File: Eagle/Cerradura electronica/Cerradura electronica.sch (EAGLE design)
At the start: 19 parts, among them K1 G5L, M1 ARDUINO-NANO-3.0#ISP

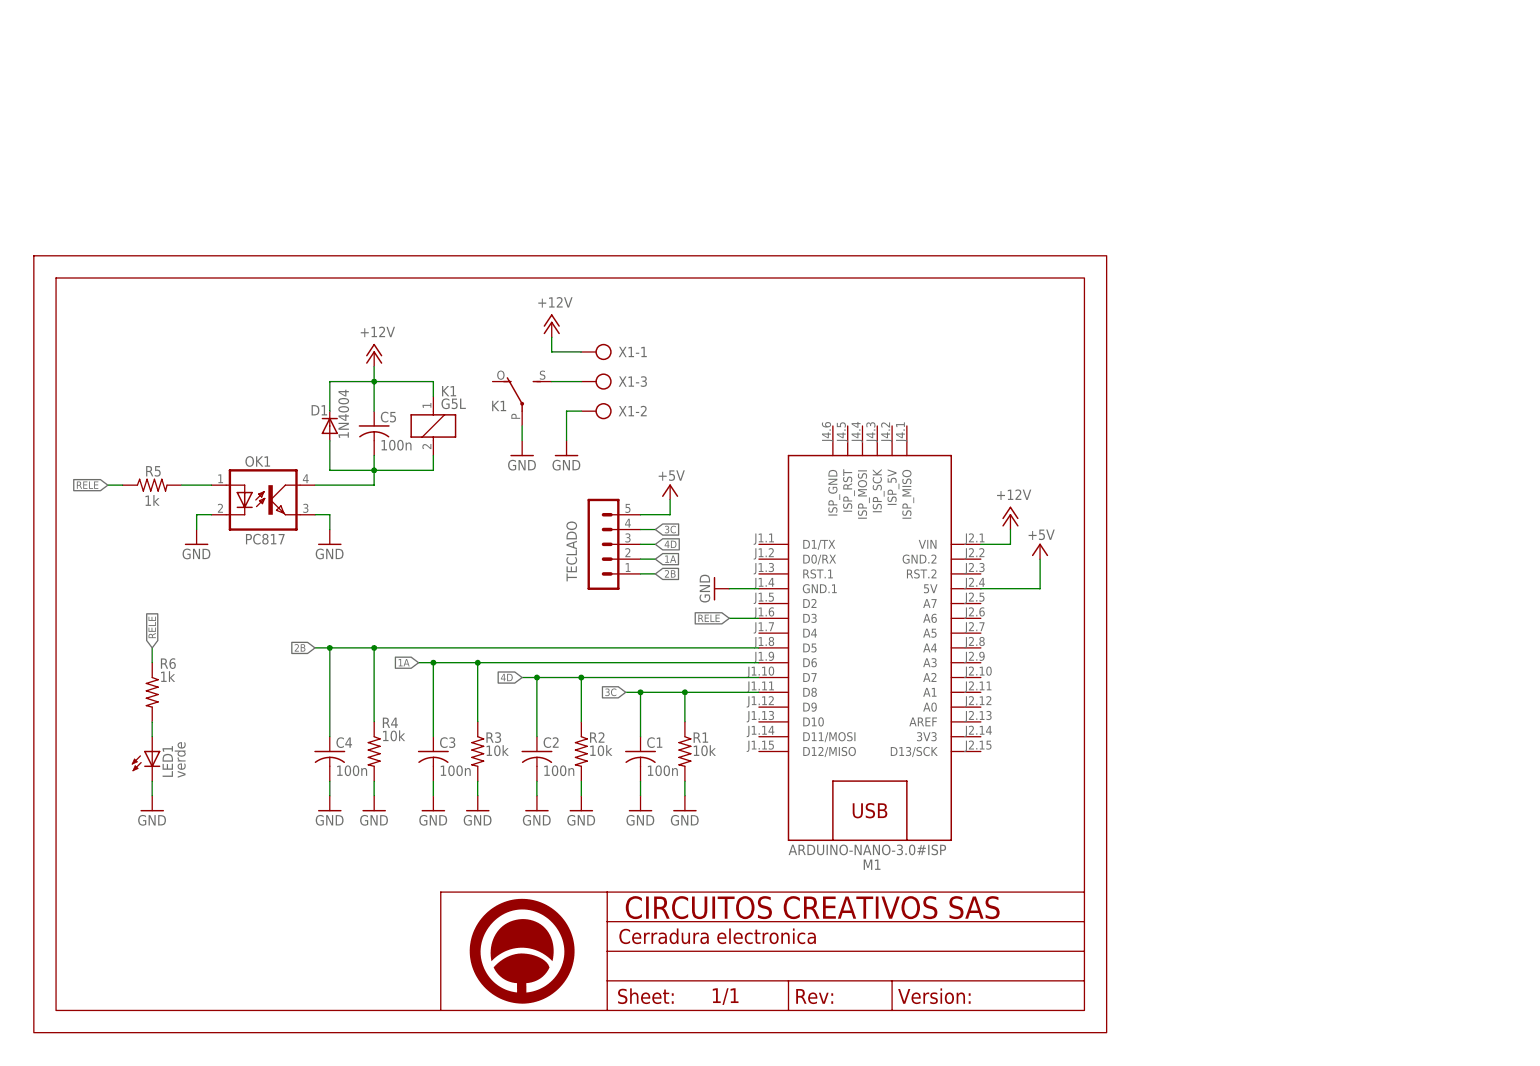
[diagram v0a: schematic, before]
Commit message: Completado SCH del nuevo Hardware al 50%
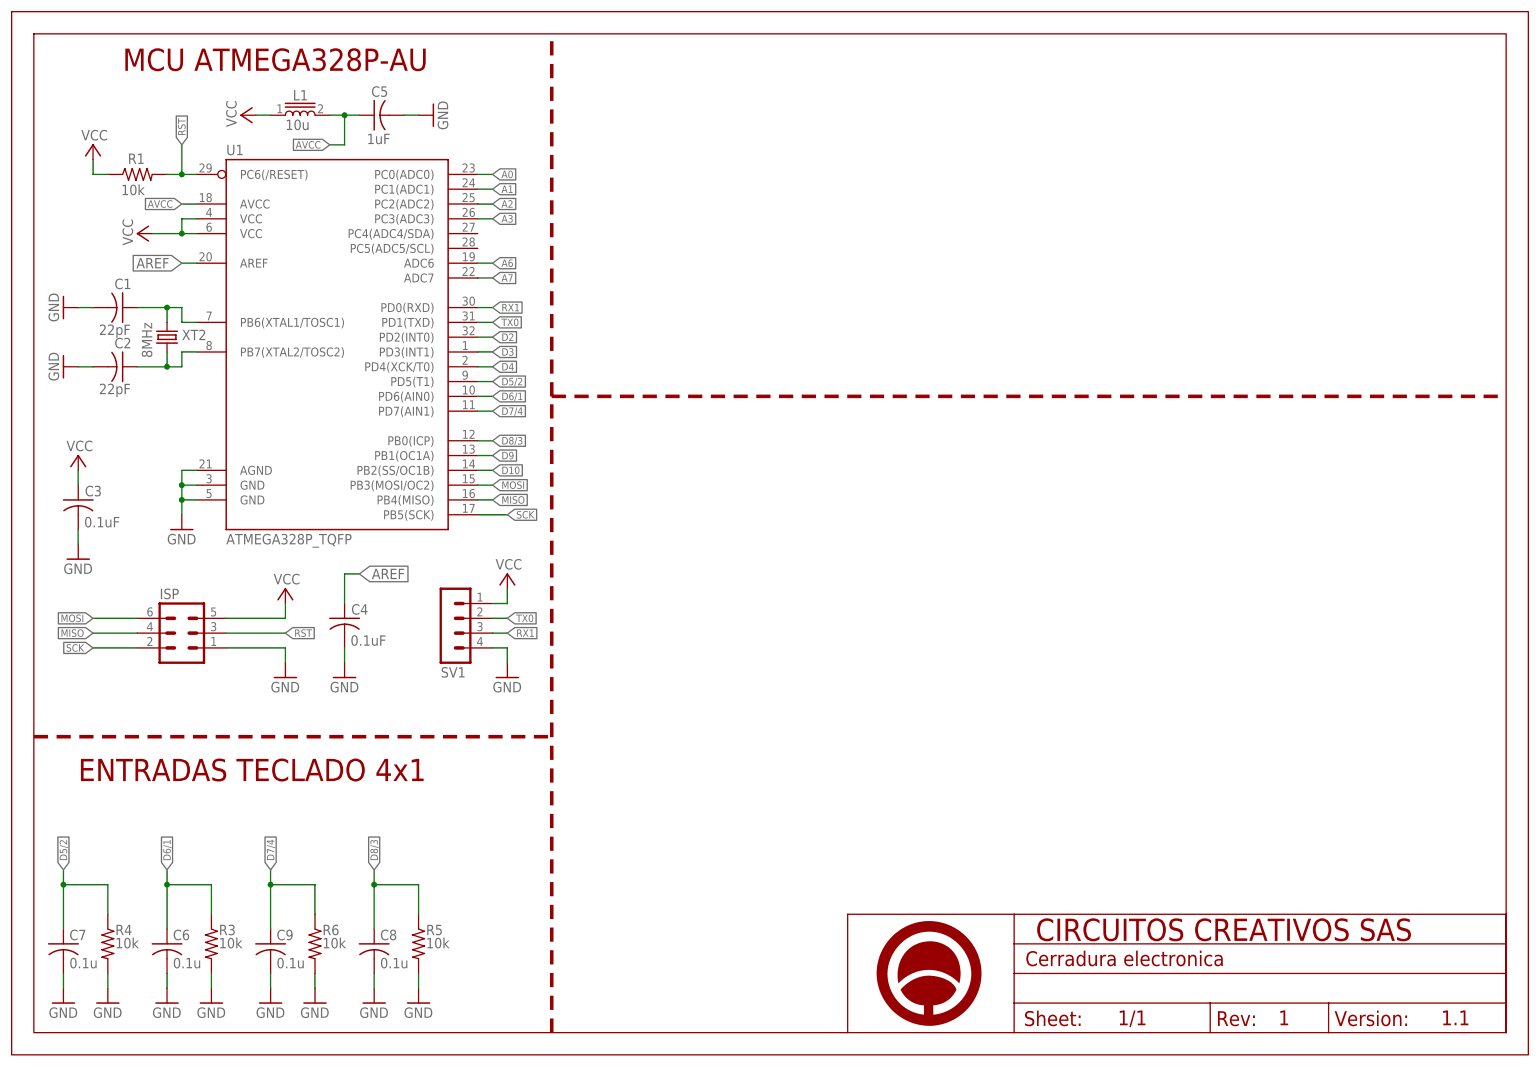
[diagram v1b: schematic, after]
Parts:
- removed D1: 1N4004, adafruit:1N4004
- removed K1: G5L, relay:G5L
- removed LED1: verde, led:LED3MM
- removed M1: ARDUINO-NANO-3.0#ISP, DIY- comercial modules:ARDUINO-NANO-3.0#ISP
- removed OK1: PC817, optocoupler:PC817
- removed R2: 10k, rcl:R-US_0204/7
- removed TECLADO: (no value), con-lstb:MA05-1
- removed X1: (no value), con-ptr500:AK500/3
- added C6, C7, C8, C9: 0.1u, rcl:C-USC0805
- added ISP: (no value), con-lstb:MA03-2
- added L1: 10u, Circuitos-Creativos-RCL:FERRITA-CHOKE
- added SV1: (no value), con-lstb:MA04-1
- added U1: ATMEGA328P_TQFP, SparkFun-DigitalIC:ATMEGA328P_TQFP
- added XT2: 8MHz, crystal:CRYSTALCTS406
- C1, C2: value 100n -> 22pF; device rcl:C-US025-025X050 -> rcl:C-USC0805
- C3, C4: value 100n -> 0.1uF; device rcl:C-US025-025X050 -> rcl:C-USC0805
- C5: value 100n -> 1uF; device rcl:C-US025-025X050 -> rcl:C-USC0805
- R1, R3, R4: device rcl:R-US_0204/7 -> rcl:R-US_R1206
- R5, R6: value 1k -> 10k; device rcl:R-US_0204/7 -> rcl:R-US_R1206
- U$1: value A5_HORIZONTAL -> A4_HORIZONTAL; device Circuitos-Creativos-Estilos:A5_HORIZONTAL -> Circuitos-Creativos-Estilos:A4_HORIZONTAL
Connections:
- removed net +12V: C5.1, D1.C, K11.1, M1.VIN, X1-1.KL
- removed net +5V: M1.5V, TECLADO.5
- removed net 1A: C3.1, M1.D6, R3.1, TECLADO.2
- removed net 2B: C4.1, M1.D5, R4.1, TECLADO.1
- removed net 3C: C1.1, M1.D8, R1.1, TECLADO.4
- removed net 4D: C2.1, M1.D7, R2.1, TECLADO.3
- removed net N$1: LED1.A, R6.2
- removed net N$2: C5.2, D1.A, K11.2, OK1.COL
- removed net N$3: OK1.A, R5.2
- removed net N$4: K12.S, X1-3.KL
- removed net RELE: M1.D3, R5.1, R6.1
- new net A0: U1.PC0(ADC0)
- new net A1: U1.PC1(ADC1)
- new net A2: U1.PC2(ADC2)
- new net A3: U1.PC3(ADC3)
- new net A6: U1.ADC6
- new net A7: U1.ADC7
- new net AREF: C4.1, U1.AREF
- new net AVCC: C5.1, L1.2, U1.AVCC
- new net D10: U1.PB2(SS/OC1B)
- new net D2: U1.PD2(INT0)
- new net D3: U1.PD3(INT1)
- new net D4: U1.PD4(XCK/T0)
- new net D5/2: C7.1, R4.1, U1.PD5(T1)
- new net D6/1: C6.1, R3.1, U1.PD6(AIN0)
- new net D7/4: C9.1, R6.1, U1.PD7(AIN1)
- new net D8/3: C8.1, R5.1, U1.PB0(ICP)
- new net D9: U1.PB1(OC1A)
- new net MISO: ISP.4, U1.PB4(MISO)
- new net MOSI: ISP.6, U1.PB3(MOSI/OC2)
- new net OS1: C1.1, U1.PB6(XTAL1/TOSC1), XT2.2
- new net OS2: C2.1, U1.PB7(XTAL2/TOSC2), XT2.1
- new net RST: ISP.3, R1.2, U1.PC6(/RESET)
- new net RX1: SV1.3, U1.PD0(RXD)
- new net SCK: ISP.2, U1.PB5(SCK)
- new net TX0: SV1.2, U1.PD1(TXD)
- new net VCC: C3.1, ISP.5, L1.1, R1.1, SV1.1, U1.VCC@4, U1.VCC@6
- net GND: now also C5.2, C6.2, C7.2, C8.2, C9.2, ISP.1, R5.2, R6.2, SV1.4, U1.AGND, U1.GND@3, U1.GND@5; no longer K12.P, LED1.C, M1.GND.1, OK1.C, OK1.EMIT, R1.2, R2.2, X1-2.KL
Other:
- note added: "1"
- note added: "1.1"
- note added: "ENTRADAS TECLADO 4x1"
- note added: "MCU ATMEGA328P-AU"
- moved on the sheet: C1, C2, C3, C4, C5, R1, R3, R4, R5, R6
